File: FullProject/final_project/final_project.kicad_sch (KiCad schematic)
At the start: 46 parts, among them J1 Conn_WallSocket, J10 Conn_01x03_Female, J2 Weight Sensor Connector, J3 PIR Array Connector 01, J4 PIR Array Connector 02, J5 PIR Array Connector 03, J6 pH Sensor Connector, J7 Keypad Connector, J8 LCD Connector, J9 Conn_01x02_Female, M1 Motor_DC, M2 Motor_Servo, Q1 2N4403, U1 L7805, U2 LM7809_TO220, U3 LM7812_TO220, U4 ATmega32A-P, U5 L293D, U7 DS3232M, U8 PCF8574

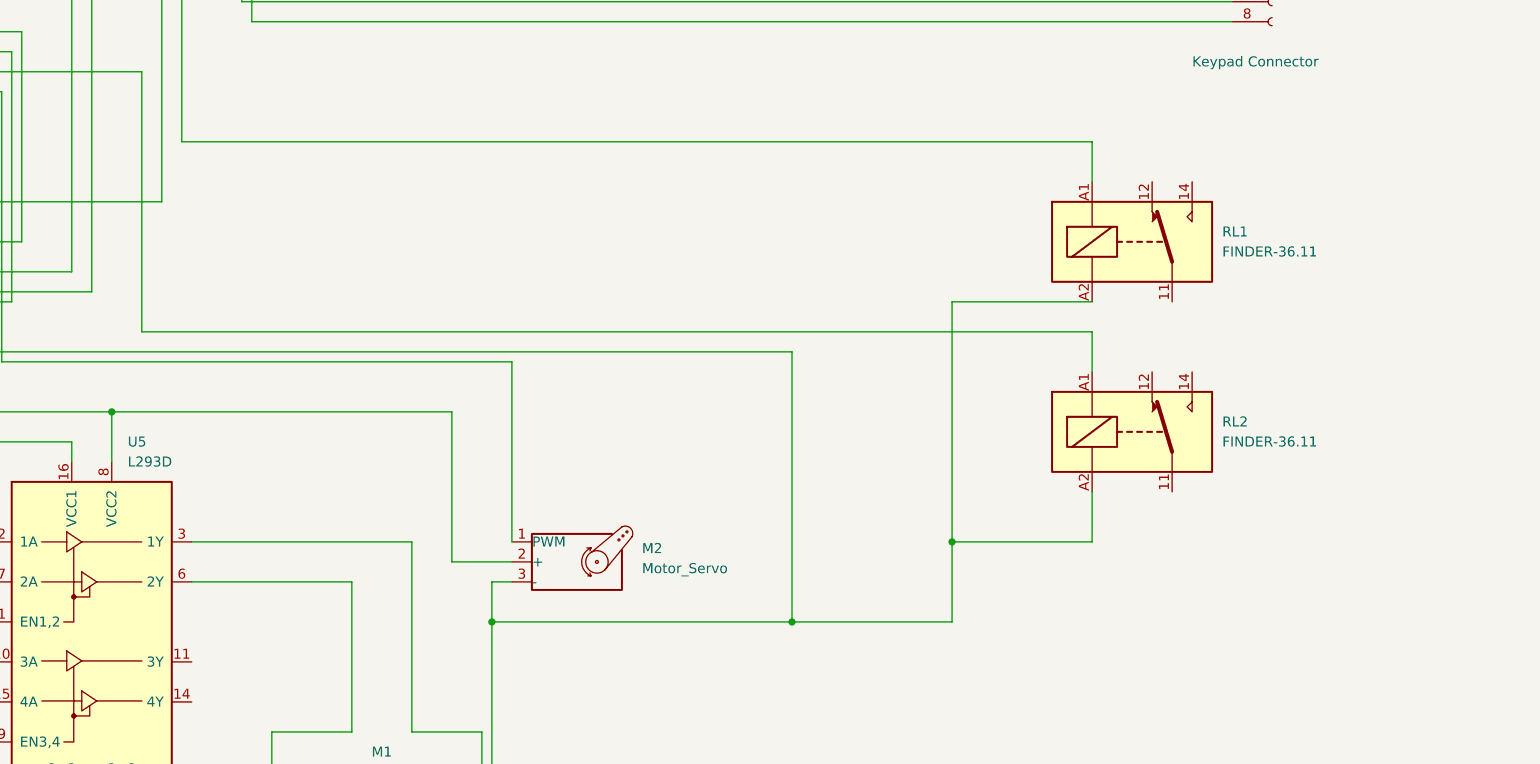
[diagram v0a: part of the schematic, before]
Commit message: add
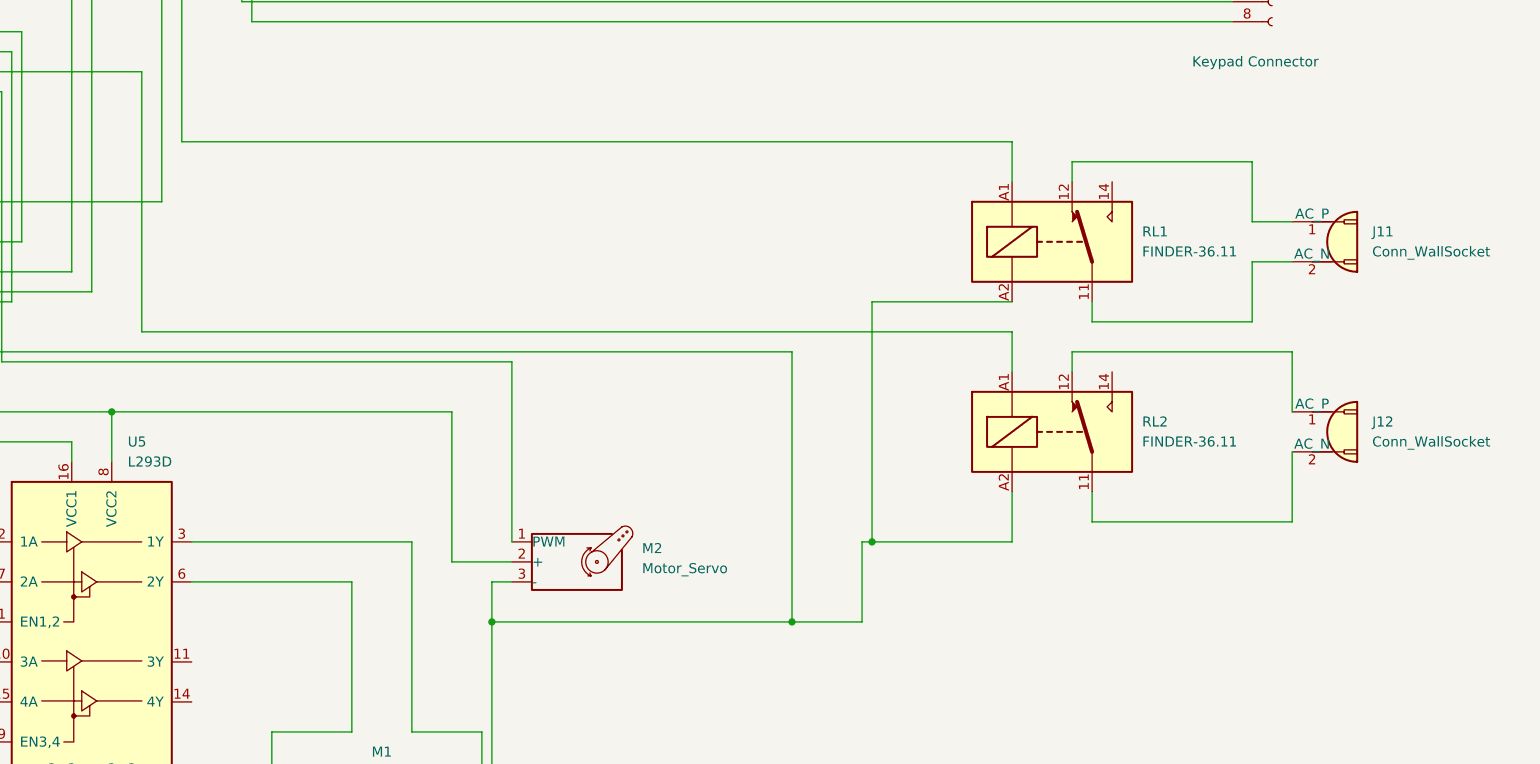
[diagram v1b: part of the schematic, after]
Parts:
- added J11, J12: Conn_WallSocket, Connector_AMASS:AMASS_XT60-M_1x02_P7.20mm_Vertical, symbol Connector:Conn_WallSocket
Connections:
- net at RL1.11: now also J11.2 (AC_N)
- net at RL1.12: now also J11.1 (AC_P)
- net at RL2.11: now also J12.2 (AC_N)
- net at RL2.12: now also J12.1 (AC_P)
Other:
- moved on the sheet: RL1, RL2

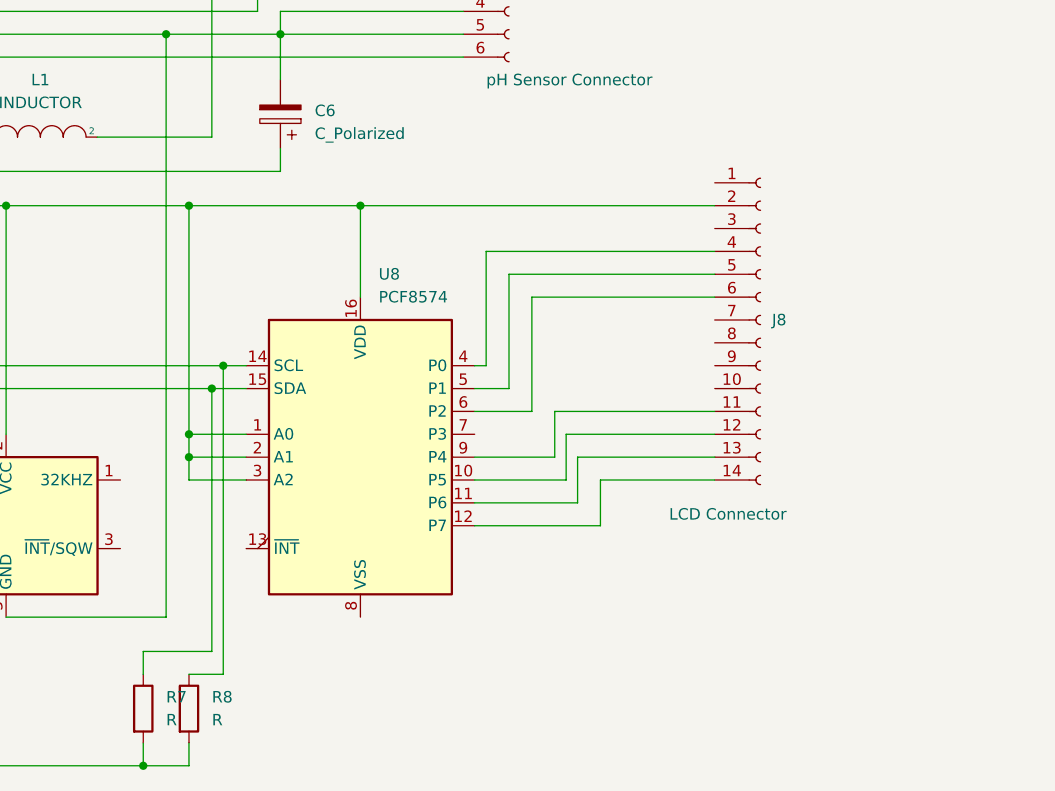
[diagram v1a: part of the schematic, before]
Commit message: add
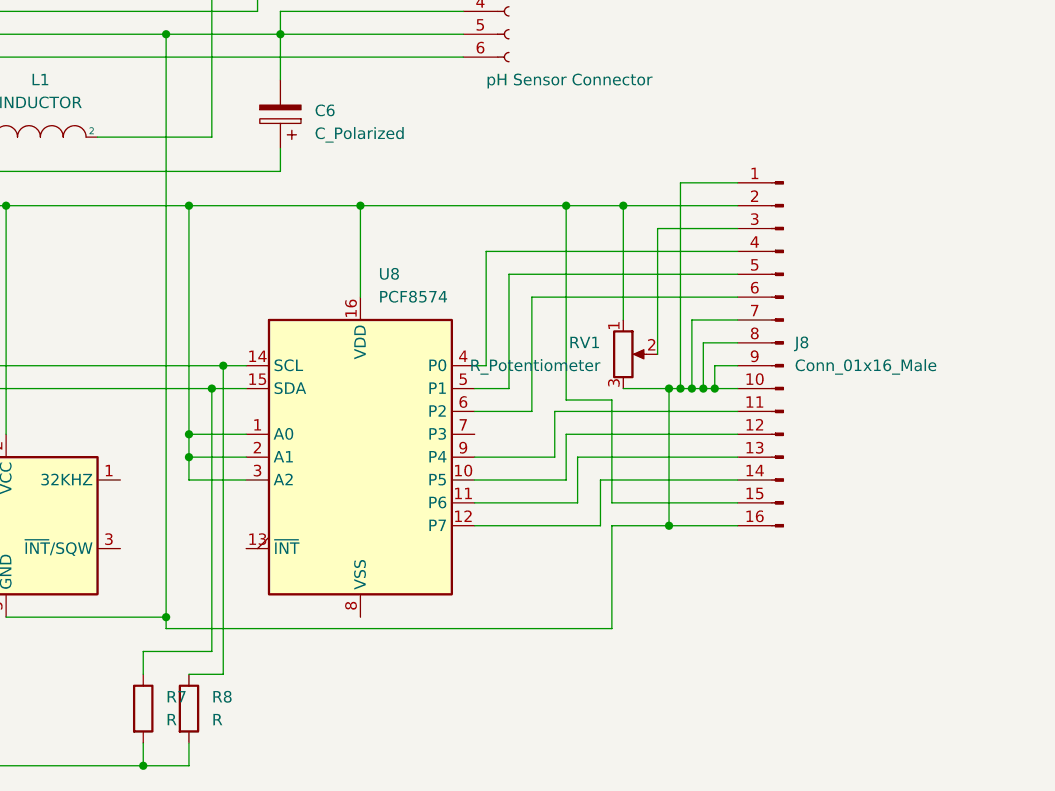
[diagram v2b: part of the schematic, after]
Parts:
- removed J8: LCD Connector, Connector_PinSocket_2.54mm:PinSocket_1x14_P2.54mm_Vertical, symbol Connector:Conn_01x14_Female
- added J8: Conn_01x16_Male, Connector_PinHeader_2.54mm:PinHeader_1x16_P2.54mm_Vertical, symbol Connector:Conn_01x16_Male
- added RV1: R_Potentiometer, Potentiometer_THT:Potentiometer_ACP_CA6-H2,5_Horizontal, symbol Device:R_Potentiometer
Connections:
- net at C3.1, HX1.1 (VSUP), HX1.16 (DVDD)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: now also J8.15 (Pin_15), J8.2 (Pin_2), RV1.1
- net at BZ1.2 (+), C1.2, C2.1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: now also J8.1 (Pin_1), J8.10 (Pin_10), J8.16 (Pin_16), J8.7 (Pin_7), J8.8 (Pin_8), J8.9 (Pin_9), RV1.3
- net at U8.10 (P5): now also J8.12 (Pin_12)
- net at U8.11 (P6): now also J8.13 (Pin_13)
- net at U8.12 (P7): now also J8.14 (Pin_14)
- net at U8.4 (P0): now also J8.4 (Pin_4)
- net at U8.5 (P1): now also J8.5 (Pin_5)
- net at U8.6 (P2): now also J8.6 (Pin_6)
- net at U8.9 (P4): now also J8.11 (Pin_11)
- new net: J8.3 (Pin_3), RV1.2
